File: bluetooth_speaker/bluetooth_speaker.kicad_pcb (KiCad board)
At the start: 2 copper layers, 70 x 44 mm, 47 parts, among them J1 Conn_Coaxial, J2 USB_C_Receptacle_USB2.0_16P, J3 282836-4, J5 Conn_01x04_Pin, Q1 SS8050-G, Q2 SS8050-G, U1 MAX98357A, U2 XL4015, U3 CP2102N-A01-GQFN28, U4 ESP32-D0WD-V3, Y1 40MHz(±10 ppm)

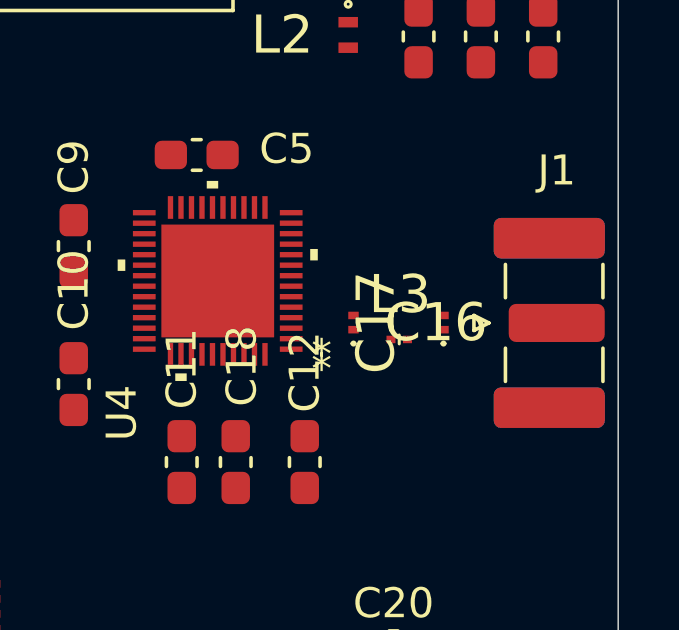
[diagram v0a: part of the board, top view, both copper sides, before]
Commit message: again
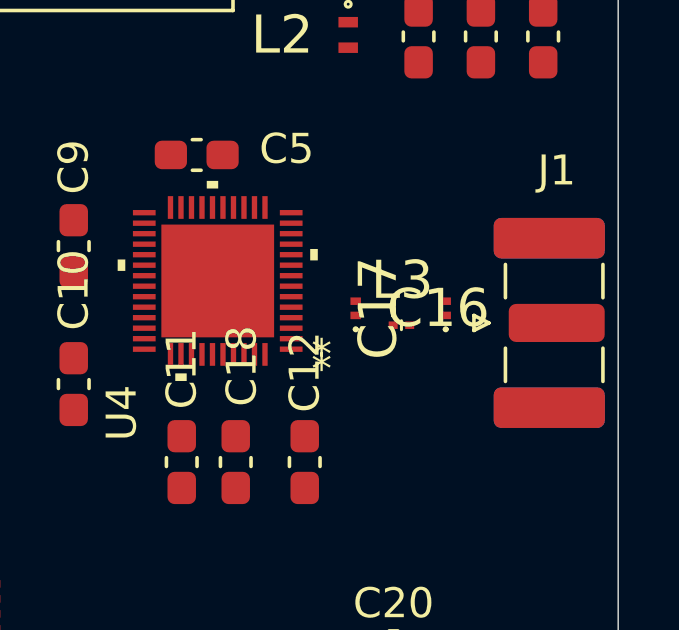
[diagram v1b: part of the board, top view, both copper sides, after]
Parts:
- moved L3 0.48 mm to (176.3, 100.6)
- moved C16 0.48 mm to (174.8, 100.0)
- moved C17 0.48 mm to (177.8, 100.0)
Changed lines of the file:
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@@
 	(footprint "SamacSys_Parts:LQP03TG3N1B02D"
 		(layer "F.Cu")
-		(at 176.2013 101.075)
+		(at 176.275 100.6)
 		(descr "0201 (0603) T=0.3±0.03mm")
 		(tags "Inductor")
@@
 	(footprint "SamacSys_Parts:GRM033D70J224ME01D"
 		(layer "F.Cu")
-		(at 174.6763 100.512 90)
+		(at 174.75 100.037 90)
 		(descr "GRM03")
 		(tags "Capacitor")
@@
 	(footprint "SamacSys_Parts:GRM033D70J224ME01D"
 		(layer "F.Cu")
-		(at 177.6763 100.512 90)
+		(at 177.75 100.037 90)
 		(descr "GRM03")
 		(tags "Capacitor")
@@
 	)
 	(segment
+		(start 181.525 100.525)
+		(end 181.6 100.6)
+		(width 0.15)
+		(layer "F.Cu")
+		(net 5)
+	)
+	(segment
+		(start 181.4513 100.525)
+		(end 181.525 100.525)
+		(width 0.15)
+		(layer "F.Cu")
+		(net 5)
+	)
+	(segment
